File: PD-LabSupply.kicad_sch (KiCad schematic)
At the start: 86 parts, among them J1 Conn_01x02, J2 Conn_02x02_Odd_Even, J3 USB_C_Receptacle_USB2.0, J6 Conn_01x07, Q1 BC847, Q4 IRF9393, SW1 SW_DIP_x06, SW2 SW_DPST_x2, SW3 SW_Push, SW4 SW_Push, SW5 SW_DPST_x2, SW6 SW_Push, SW7 SW_Push, U1 SRV05-4, U3 TMCS1108, U4 AP33772, U5 RP2040, U6 oledSym, U7 LMR54410, U8 AP2112K-3.3TRG1, U9 W25Q16JVSSIQ, Y1 Crystal_GND24

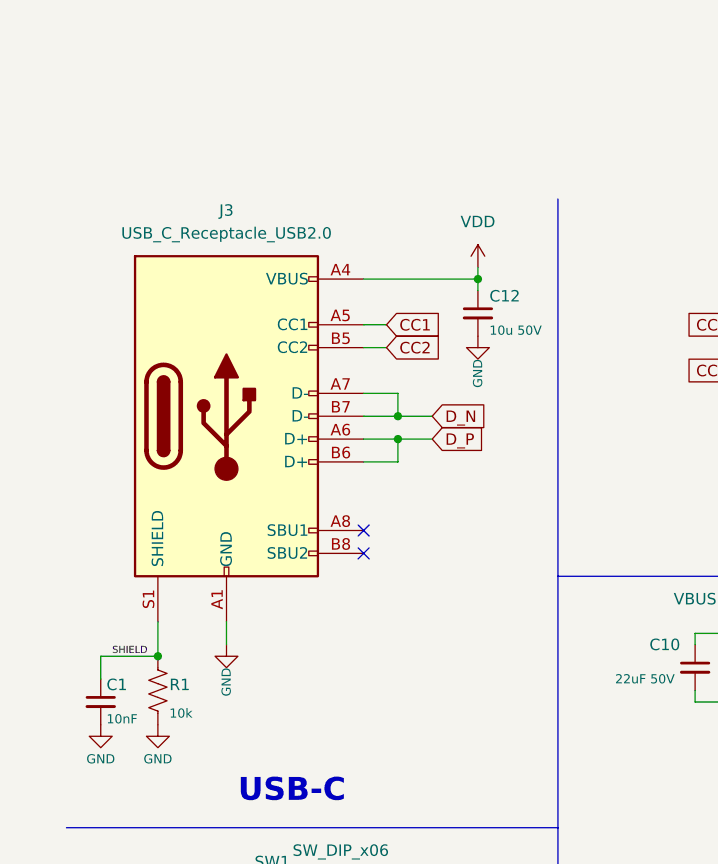
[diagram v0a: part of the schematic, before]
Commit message: fertig
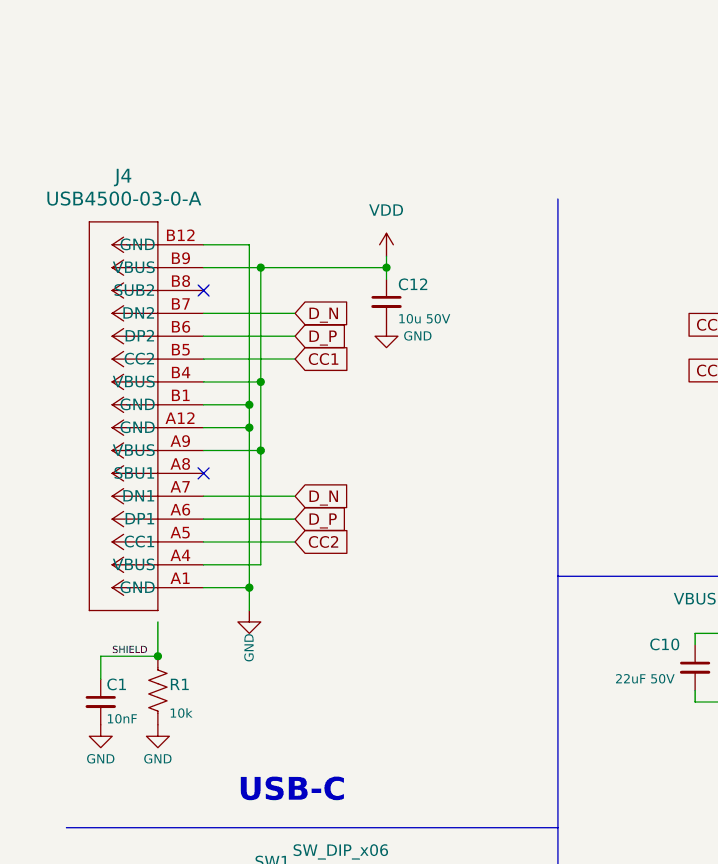
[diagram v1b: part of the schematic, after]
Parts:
- removed J3: USB_C_Receptacle_USB2.0, Connector_USB:USB_C_Receptacle_JAE_DX07S016JA1R1500, symbol Connector:USB_C_Receptacle_USB2.0
- added J4: USB4500-03-0-A, USB4500_03_0_A:CONN_USB4500_GCT, symbol USB4500_03_0_A:USB4500-03-0-A
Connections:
- net CC1: now also J4.B5 (CC2)
- net CC2: now also J4.A5 (CC1)
- net D_N: now also J4.A7 (DN1), J4.B7 (DN2)
- net D_P: now also J4.A6 (DP1), J4.B6 (DP2)
- net GND: now also J4.A1 (GND), J4.A12 (GND), J4.B1 (GND), J4.B12 (GND)
- net VDD: now also J4.A4 (VBUS), J4.A9 (VBUS), J4.B4 (VBUS), J4.B9 (VBUS)
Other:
- moved on the sheet: C12
